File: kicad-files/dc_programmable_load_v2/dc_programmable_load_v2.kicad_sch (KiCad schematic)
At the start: 43 parts, among them J1 DC Jack 12V, J3 Conn_01x04_Socket, Q1 IRF3205, U1 LM358DR, U2 ER_OLEDM0.91_1x-I2C, U3 AP63200WU, U4 DS18B20, U5 S-2050

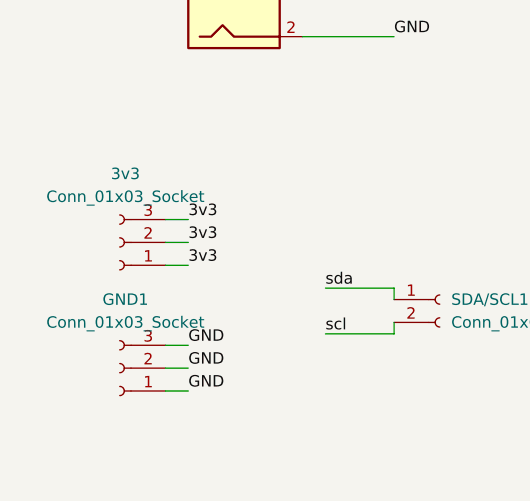
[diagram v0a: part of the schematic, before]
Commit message: Update v2 design files and m1_key PCB
Co-Authored-By: Claude Opus 4.8 (1M context) <noreply@anthropic.com>
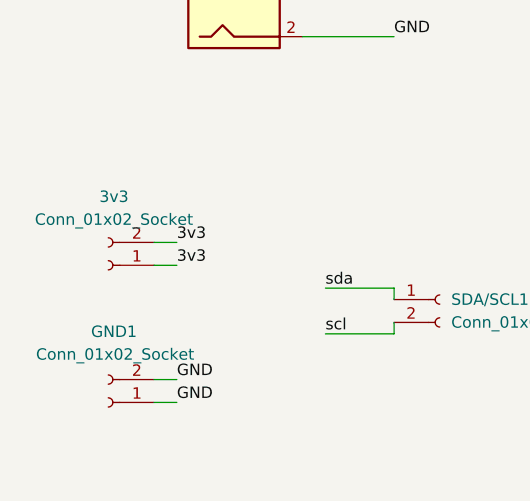
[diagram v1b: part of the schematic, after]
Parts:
- removed 3v3, GND1: Conn_01x03_Socket, Connector_PinHeader_2.00mm:PinHeader_1x03_P2.00mm_Vertical, symbol Connector:Conn_01x03_Socket
- added 3v3, GND1: Conn_01x02_Socket, Connector_PinHeader_2.54mm:PinHeader_1x02_P2.54mm_Vertical, symbol Connector:Conn_01x02_Socket
- J3: footprint Connector_PinHeader_2.00mm:PinHeader_1x04_P2.00mm_Vertical -> Connector_PinHeader_2.54mm:PinHeader_1x04_P2.54mm_Vertical
- Res1, Res2, SDA/SCL1: footprint Connector_PinHeader_2.00mm:PinHeader_1x02_P2.00mm_Vertical -> Connector_PinHeader_2.54mm:PinHeader_1x02_P2.54mm_Vertical
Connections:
- net 3v3: now also 3v3.1 (Pin_1), 3v3.2 (Pin_2)
- net GND: now also GND1.1 (Pin_1), GND1.2 (Pin_2)
